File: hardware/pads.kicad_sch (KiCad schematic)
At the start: 60 parts, among them CN1 SM04B-SRSS-TB, J1 5V, J10 5V, J11 5V, J12 5V, J13 5V, J14 5V, J15 5V, J16 5V, J17 5V, J18 5V, J19 5V, J2 5V, J20 5V, J21 5V, J22 5V, J23 5V, J24 5V, J25 5V, J26 5V, J27 5V, J28 5V, J29 5V, J3 5V, J30 5V, J31 5V, J32 5V, J33 5V, J34 5V, J35 5V, J36 5V, J37 5V, J38 5V, J39 5V, J4 5V, J40 5V, J41 5V, J42 5V, J43 5V, J44 5V, J45 5V, J46 5V, J47 5V, J48 5V, J49 5V, J5 5V, J50 5V, J51 5V, J52 5V, J53 5V, J54 5V, J55 5V, J6 5V, J7 5V, J8 5V, J9 5V, P1 SM08B-SRSS-TB(LF)(SN), U13 SM03B-SRSS-TB, U14 SM06B-SRSS-TB(LF)(SN), U8 SM06B-SRSS-TB(LF)(SN)

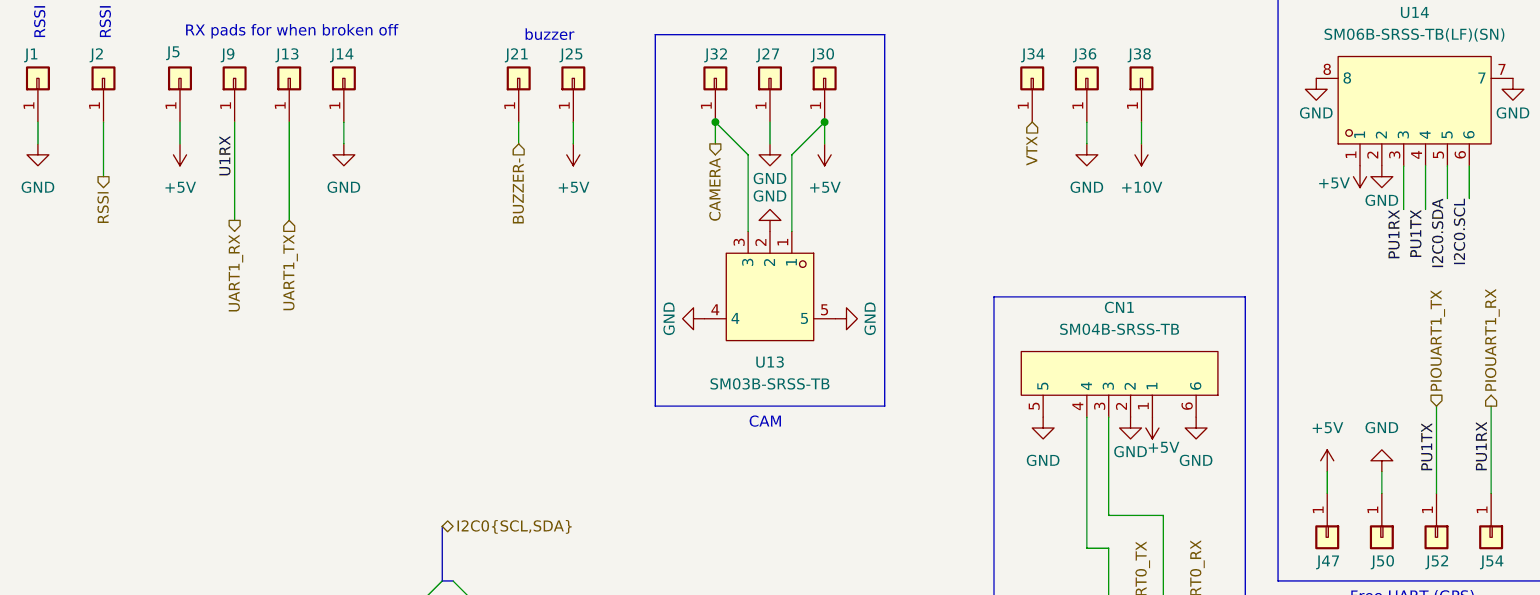
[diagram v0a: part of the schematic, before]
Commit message: ok
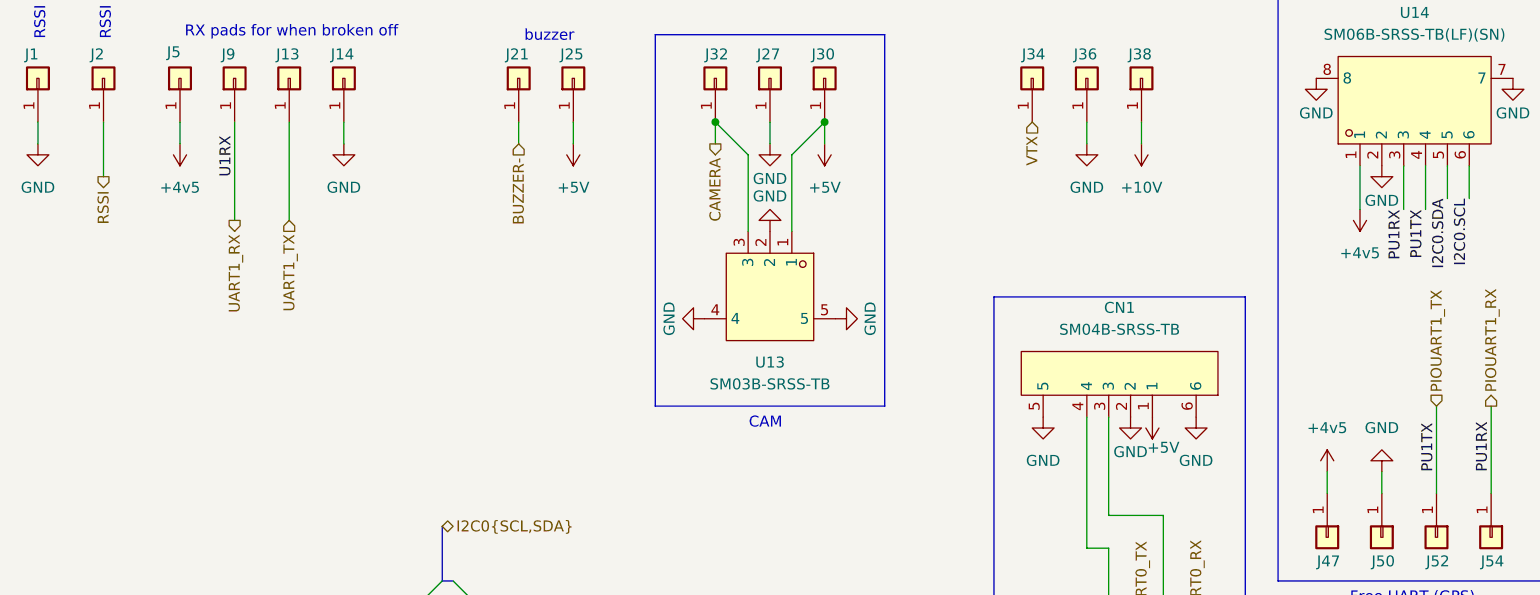
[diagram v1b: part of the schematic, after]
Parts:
- CN1: LCSC (none) -> C160404; LCSC Part C160404 -> (none)
- J10, J16, J19, J23, J3, J6: now left out of the parts list
- U13: LCSC (none) -> C160403; LCSC Part C160403 -> (none)
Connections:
- net +5V: no longer J47.1 (Pin_1), J5.1 (Pin_1), U14.1
- new net +4v5: J47.1 (Pin_1), J5.1 (Pin_1), U14.1
